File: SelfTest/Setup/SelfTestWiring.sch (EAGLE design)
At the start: 15 parts

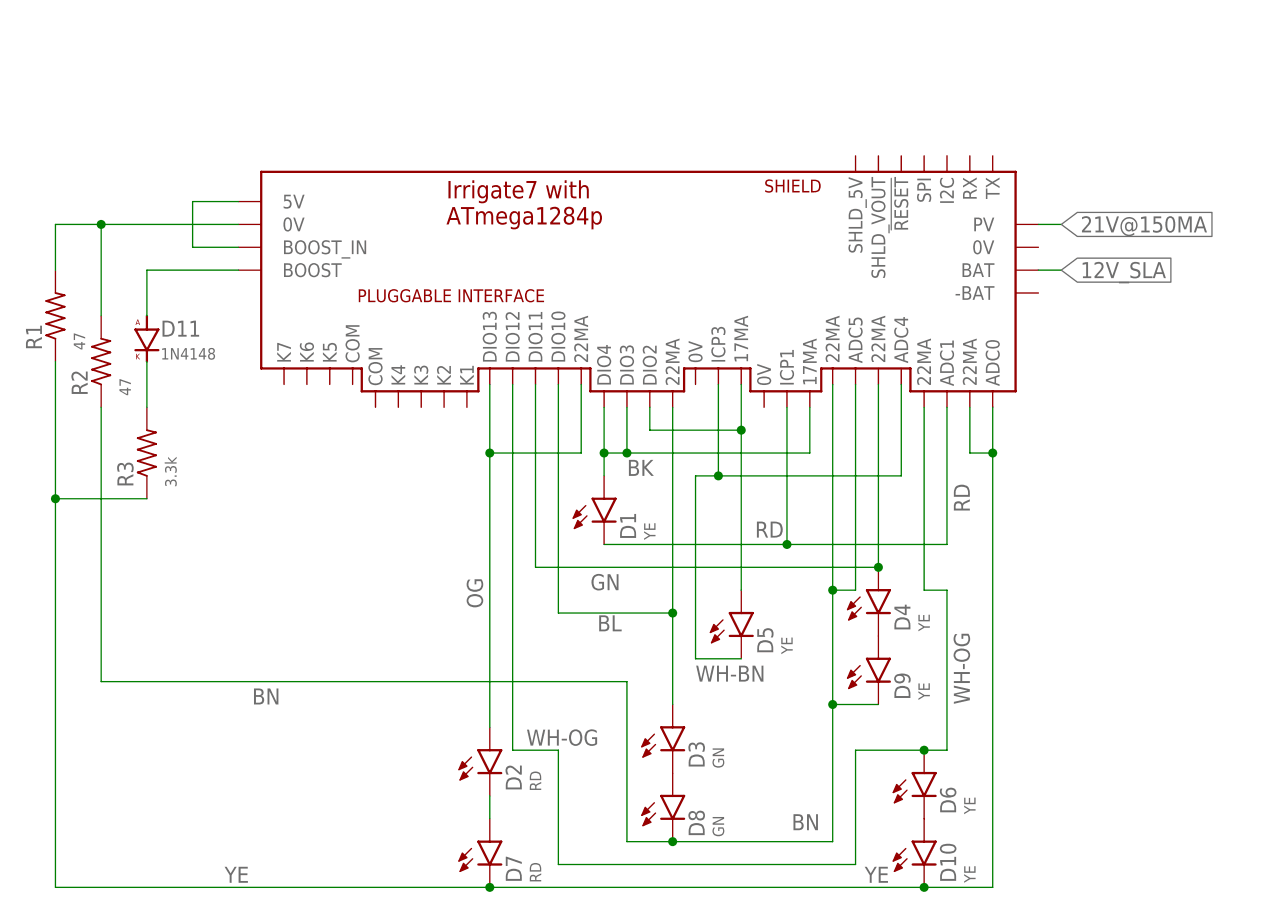
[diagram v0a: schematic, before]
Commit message: BlinkLED: updates for ^5
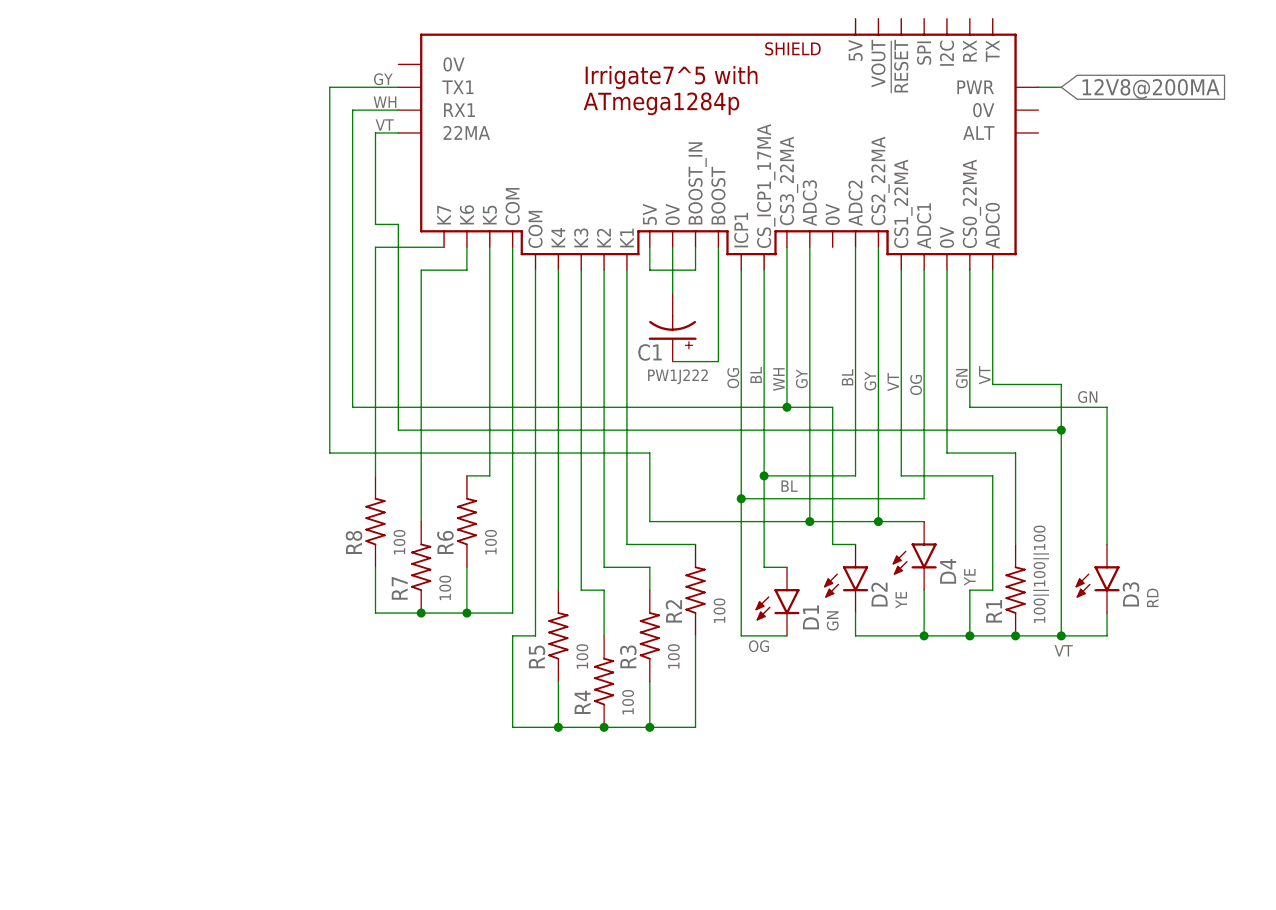
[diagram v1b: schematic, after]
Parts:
- removed D10, D5, D6, D9: YE, D-LED:LED5MM
- removed D11: 1N4148, D-GP:DDO41-10
- removed D7: RD, D-LED:LED5MM
- removed D8: GN, D-LED:LED5MM
- removed U$1: IRRIGATE7, Documentation:IRRIGATE7
- added C1: PW1J222, C-Al:C-AL7.5X18
- added R4, R5, R6, R7, R8: 100, R-C:R0805
- added U$2: IRRIGATE7, Documentation:IRRIGATE7
- D1: value YE -> GN
- D2: value RD -> YE
- D3: value GN -> RD
- R1: value 47 -> 100||100||100
- R2: value 47 -> 100
- R3: value 3.3k -> 100
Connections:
- removed net 12V_SLA: U$1.BAT
- removed net 21V@150MA: U$1.PV
- removed net BK: D1.A, U$1.17MA@ICP1, U$1.DIO3, U$1.DIO4
- removed net BN: D8.K, D9.K, R2.1, U$1.22MA@ADC5, U$1.ADC5
- removed net N$14: D10.A, D6.K
- removed net N$15: D3.K, D8.A
- removed net N$18: D4.K, D9.A
- removed net RD: D1.K, U$1.ADC1, U$1.ICP1
- removed net WH-BN: D5.K, U$1.ADC4, U$1.ICP3
- removed net WH-OG: D6.A, U$1.22MA@ADC1, U$1.DIO12
- removed net YE: D10.K, D7.K, R1.1, R3.1, U$1.22MA@ADC0, U$1.ADC0
- new net 12V8@200MA: U$2.PWR
- new net GY: D4.A, U$2.ADC3, U$2.CS2_22MA, U$2.TX1
- new net N$10: C1.-, U$2.0V
- new net N$12: R7.2, U$2.K6
- new net N$5: R5.2, U$2.K4
- new net N$6: R4.2, U$2.K3
- new net N$7: R3.2, U$2.K2
- new net N$8: R6.2, U$2.K5
- new net N$9: R6.1, R7.1, R8.1, U$2.COM@K5
- new net VT: D2.K, D3.K, D4.K, R1.1, U$2.22MA@IO, U$2.ADC0, U$2.CS1_22MA
- new net WH: D2.A, U$2.CS3_22MA, U$2.RX1
- net BL: now also D1.A, U$2.ADC2, U$2.CS_ICP1_17MA; no longer D3.A, U$1.22MA@DIO2, U$1.DIO10
- net GN: now also D3.A, U$2.CS0_22MA; no longer D4.A, U$1.22MA@ADC4, U$1.DIO11
- net N$1: now also U$2.5V, U$2.BOOST_IN; no longer U$1.5V, U$1.BOOST_IN
- net N$11: now also C1.+, U$2.BOOST; no longer D5.A, U$1.17MA@ICP3, U$1.DIO2
- net N$13: now also R8.2, U$2.K7; no longer D2.K, D7.A
- net N$2: now also R2.2, U$2.K1; no longer D11.A, U$1.BOOST
- net N$3: now also R2.1, R3.1, R4.1, R5.1, U$2.COM@K4; no longer D11.K, R3.2
- net N$4: now also U$2.0V@ADC0; no longer R2.2, U$1.0V
- net OG: now also D1.K, U$2.ADC1, U$2.ICP1; no longer D2.A, U$1.22MA@DIO10, U$1.DIO13
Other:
- note added: "240mA@24V IS 5.76W PULSE 50mSec"
- note added: "C1 2200uF 63V 3.2A RPPL 18ODx40H mm"
- note removed: "BOOST OUTPUT IS SET WITH A JUMPER AT 9V R1 HAS 2.7mA AT 12V R1 HAS 3.6mA AT 24V R1 HAS 7.2mA DIO13 LOW, OTHER CURR SOURCES ARE OFF"
- moved on the sheet: D1, D2, D3, D4, R1, R2, R3
